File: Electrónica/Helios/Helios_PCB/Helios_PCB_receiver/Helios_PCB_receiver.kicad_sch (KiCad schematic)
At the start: 11 parts, among them J0 Connector, U0 OPA2380, U1 OPA2380

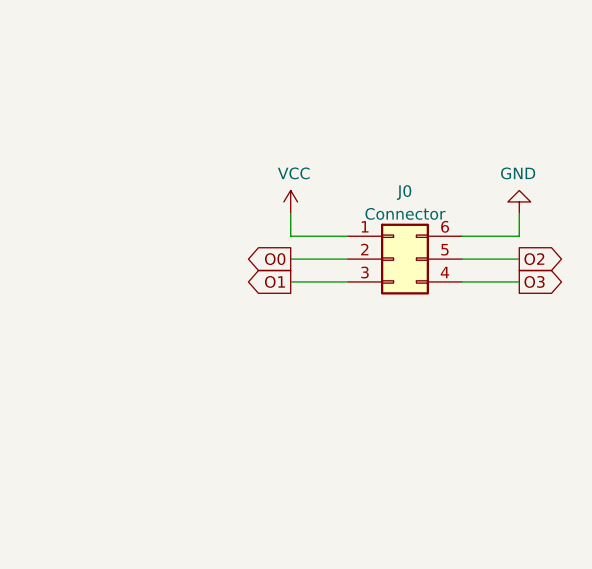
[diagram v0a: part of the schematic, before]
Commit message: Helios Panel
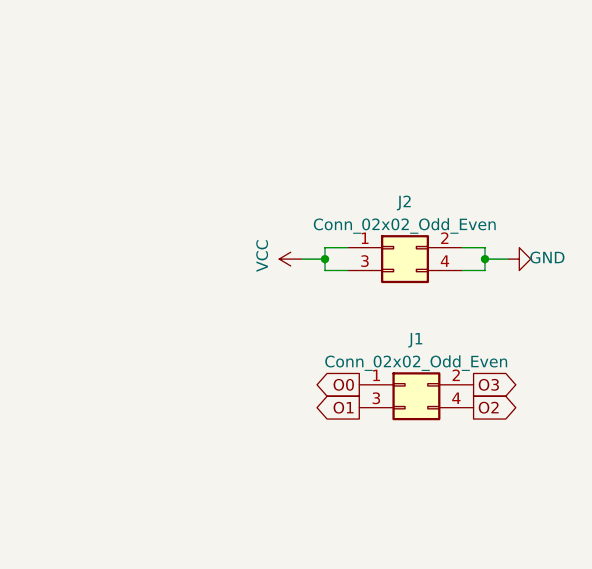
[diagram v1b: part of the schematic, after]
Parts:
- removed J0: Connector, Connector_PinHeader_2.54mm:PinHeader_2x03_P2.54mm_Vertical, symbol Connector_Generic:Conn_02x03_Counter_Clockwise
- added J1, J2: Conn_02x02_Odd_Even, Connector_PinHeader_2.54mm:PinHeader_2x02_P2.54mm_Vertical, symbol Connector_Generic:Conn_02x02_Odd_Even
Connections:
- net GND: now also J2.2 (Pin_2), J2.4 (Pin_4)
- net O0: now also J1.1 (Pin_1)
- net O1: now also J1.3 (Pin_3)
- net O2: now also J1.4 (Pin_4)
- net O3: now also J1.2 (Pin_2)
- net VCC: now also J2.1 (Pin_1), J2.3 (Pin_3)
